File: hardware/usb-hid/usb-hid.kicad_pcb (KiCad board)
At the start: 2 copper layers, 40.9 x 44.5 mm, 38 parts, among them J1 PC_USB, J2 Debug_UART, J3 MCU_SWD, J4 Ext_Power, J5 Extra-IO-2, J6 Extra-IO-1, J7 Conn_01x02_Female, J8 Extra-IO-0, SW1 E_SW, SW2 Reset, SW3 Boot, SW4 Power_SW, U1 AMS1117-3.3, U2 STM32F103C8, U3 NRF24L01_SMD, Y1 Crystal

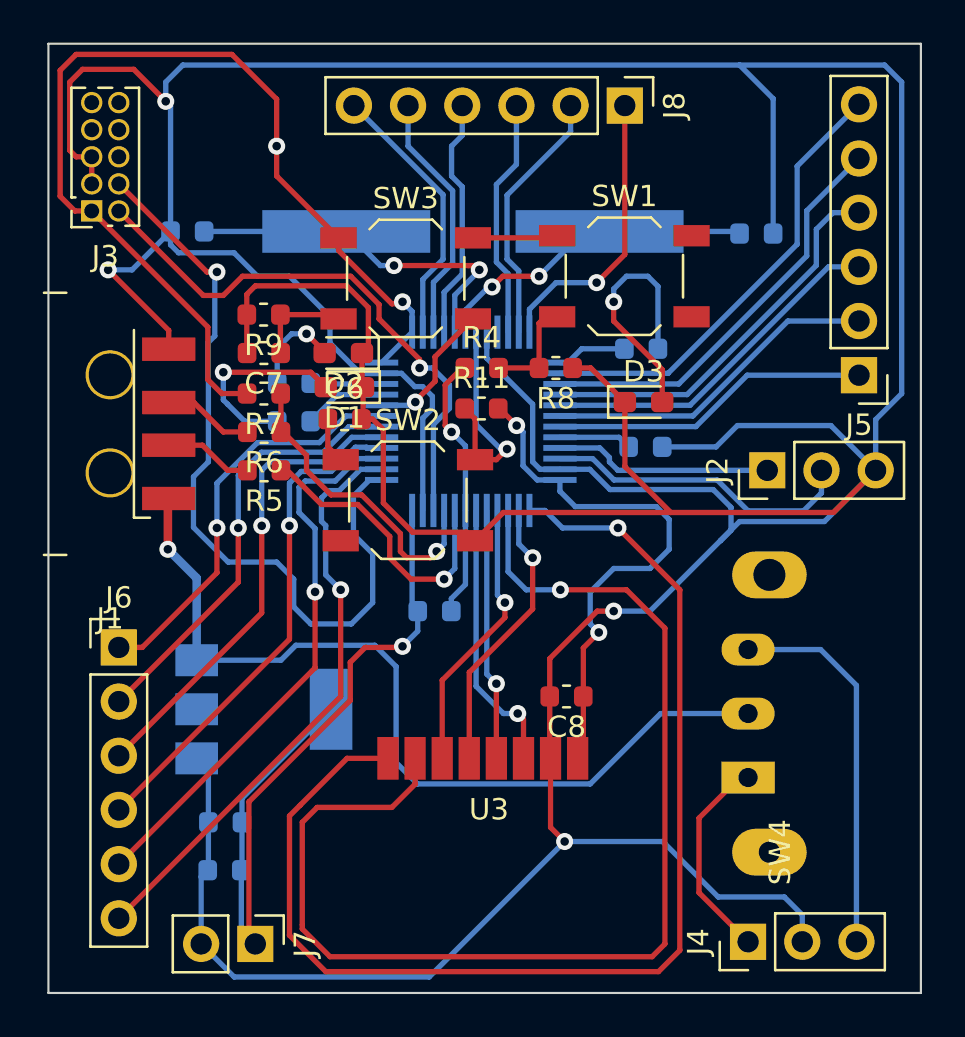
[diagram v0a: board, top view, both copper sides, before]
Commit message: Move components
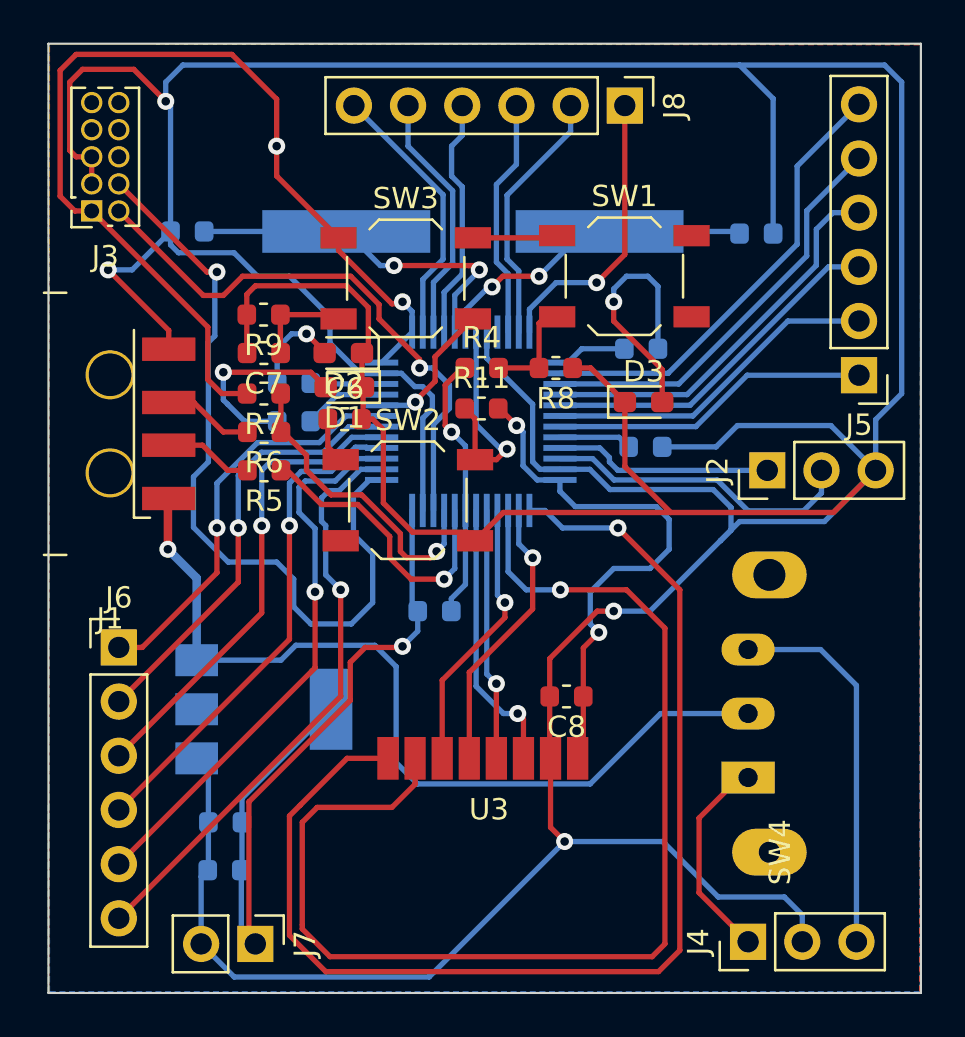
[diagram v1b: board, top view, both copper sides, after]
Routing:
- added copper zone on B.Cu, net GND
- added copper zone on F.Cu, net GND
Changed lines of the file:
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@@
   (page A4)
   (layers
-    (0 F.Cu signal)
+    (0 F.Cu signal hide)
     (31 B.Cu signal)
     (32 B.Adhes user hide)
-    (33 F.Adhes user hide)
-    (34 B.Paste user)
-    (35 F.Paste user hide)
+    (33 F.Adhes user)
+    (34 B.Paste user hide)
+    (35 F.Paste user)
     (36 B.SilkS user hide)
-    (37 F.SilkS user hide)
-    (38 B.Mask user)
-    (39 F.Mask user hide)
-    (40 Dwgs.User user)
+    (37 F.SilkS user)
+    (38 B.Mask user hide)
+    (39 F.Mask user)
+    (40 Dwgs.User user hide)
     (41 Cmts.User user)
     (42 Eco1.User user)
@@
     (44 Edge.Cuts user)
     (45 Margin user)
-    (46 B.CrtYd user)
+    (46 B.CrtYd user hide)
     (47 F.CrtYd user)
     (48 B.Fab user hide)
@@
   (segment (start 60.8 63.4) (end 62.8 63.4) (width 0.25) (layer B.Cu) (net 50))
   (segment (start 59.78 64.05) (end 60.15 64.05) (width 0.25) (layer B.Cu) (net 50))
+  (zone (net 1) (net_name GND) (layer B.Cu) (hatch edge 0.508)
+    (connect_pads (clearance 0.508))
+    (min_thickness 0.254)
+    (fill yes (arc_segments 32) (thermal_gap 0.508) (thermal_bridge_width 0.508))
+    (polygon
+      (pts
+        (xy 76.65 93.55) (xy 35.85 93.55) (xy 35.8 49.1) (xy 76.7 49.1)
+      )
+    )
+  )
+  (zone (net 1) (net_name GND) (layer F.Cu) (hatch edge 0.508)
+    (connect_pads (clearance 0.508))
+    (min_thickness 0.254)
+    (fill yes (arc_segments 32) (thermal_gap 0.508) (thermal_bridge_width 0.508))
+    (polygon
+      (pts
+        (xy 76.7 49.15) (xy 76.65 93.6) (xy 35.8 93.6) (xy 35.85 49.1)
+      )
+    )
+  )
 )
